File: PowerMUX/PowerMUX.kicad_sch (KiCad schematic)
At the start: 28 parts, among them J1 Conn_01x02_Pin, J2 UJ31-CH-G2-SMT-TR, U1 FT230XS-R, U2 LM2596S-5, U3 TPS2115APW, U4 LM3940IMP-3.3

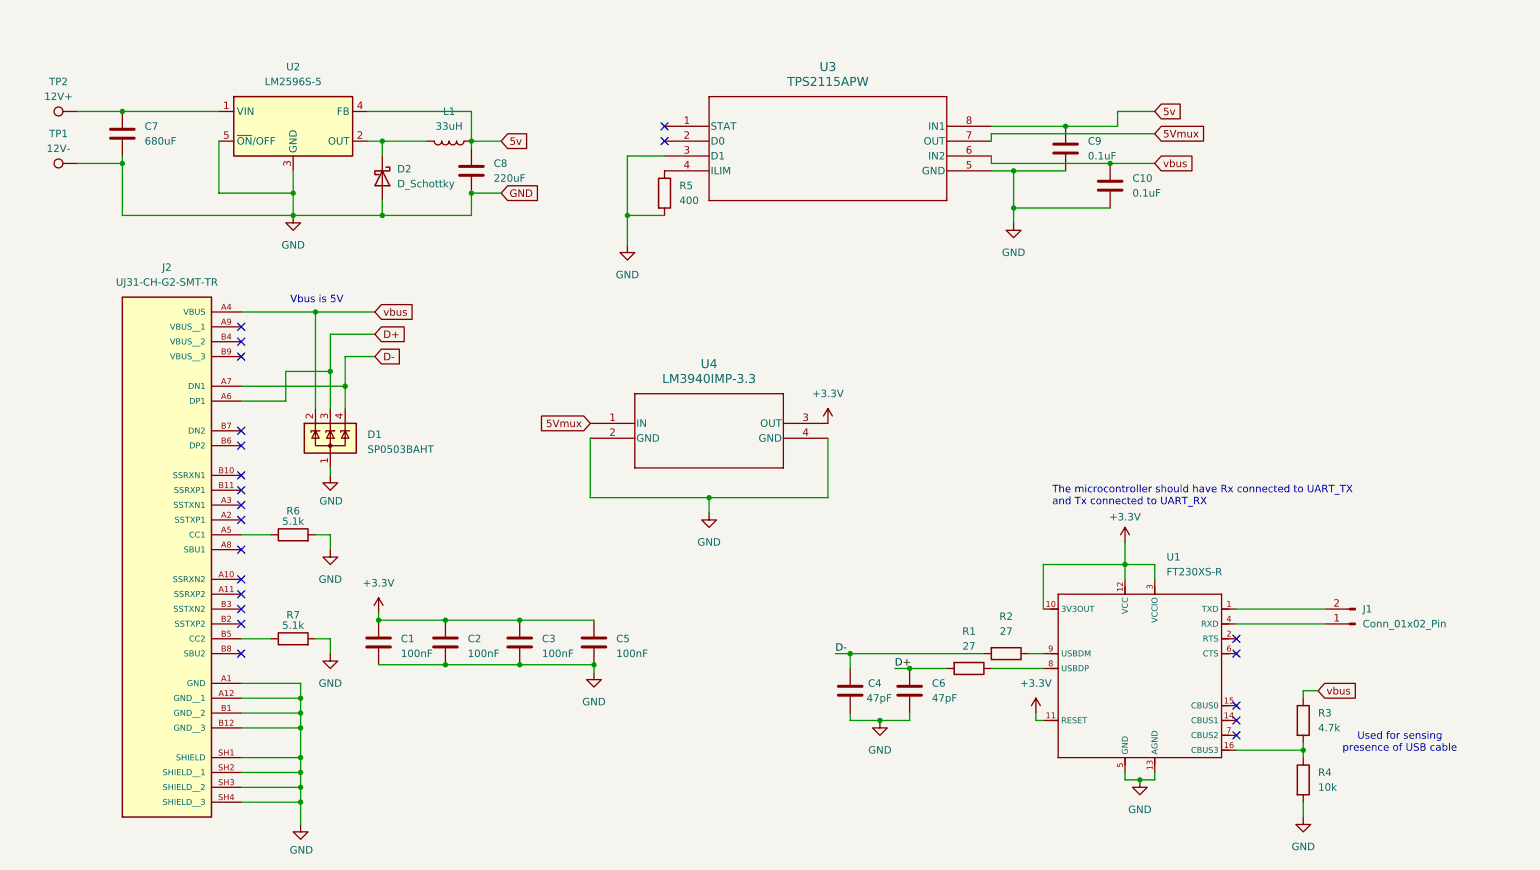
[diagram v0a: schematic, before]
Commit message: changed old THT buck converter to SMD buck converter from LSOM
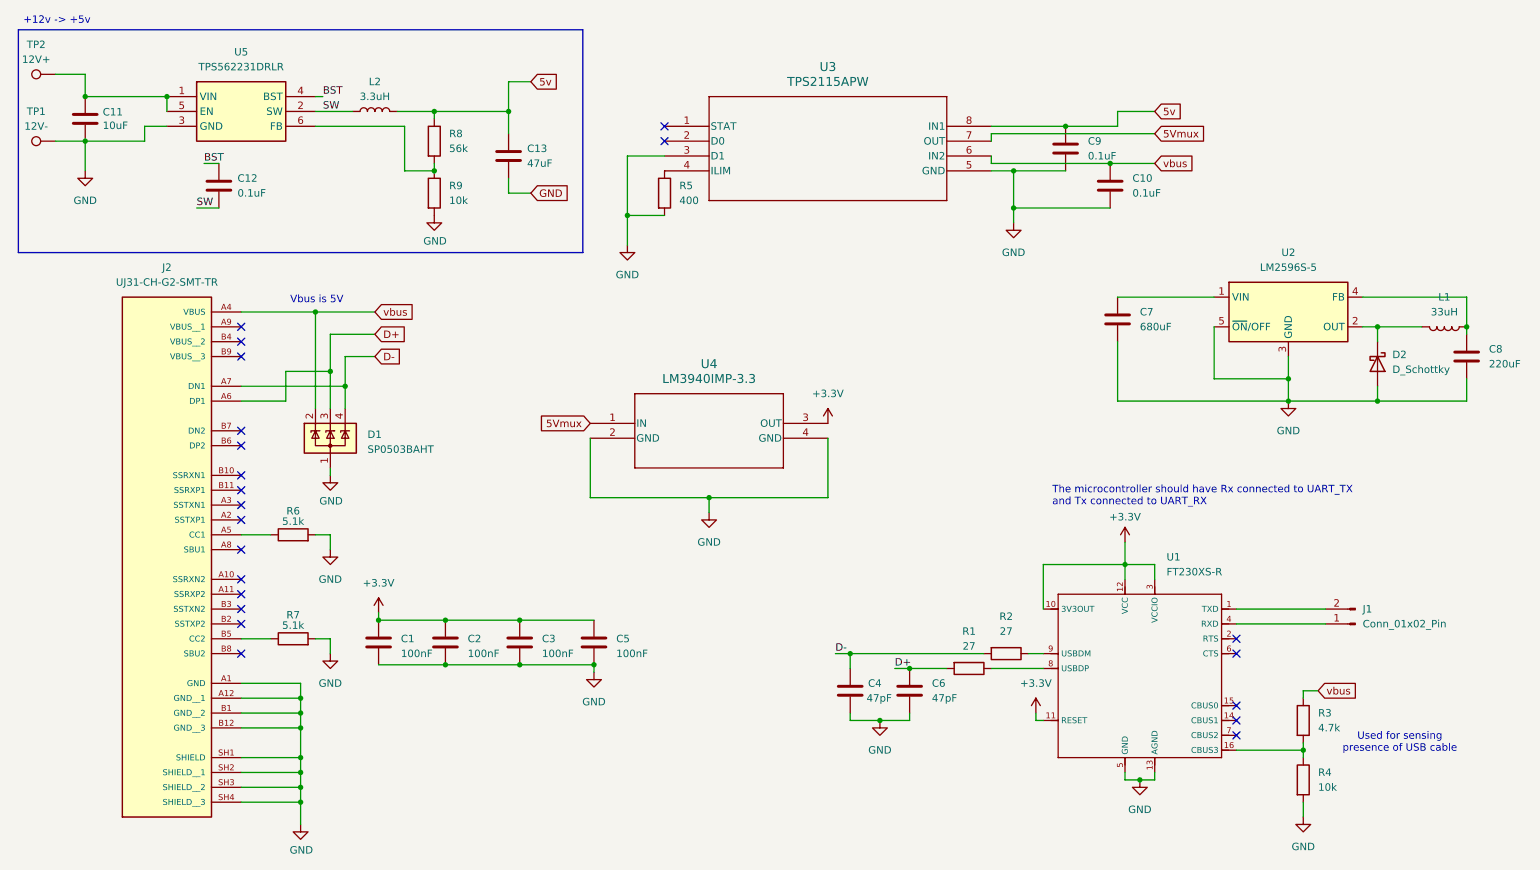
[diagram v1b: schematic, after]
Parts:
- added C11: 10uF, Capacitor_SMD:C_0805_2012Metric, symbol Device:C
- added C12: 0.1uF, Capacitor_SMD:C_0805_2012Metric, symbol Device:C
- added C13: 47uF, Capacitor_SMD:C_0805_2012Metric, symbol Device:C
- added L2: 3.3uH, Inductor_SMD:L_0805_2012Metric_Pad1.15x1.40mm_HandSolder, symbol Device:L
- added R8: 56k, Resistor_SMD:R_0805_2012Metric, symbol Device:R
- added R9: 10k, Resistor_SMD:R_0805_2012Metric, symbol Device:R
- added U5: TPS562231DRLR, Package_TO_SOT_SMD:SOT-563, symbol utsvt-power-regulators:TPS562231DRLR
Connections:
- net 5v: now also C13.1, L2.2, R8.1; no longer C8.1, L1.1, U2.4 (FB)
- net GND: now also C11.2, C13.2, R9.2, U5.3 (GND)
- net at C7.1, U2.1 (VIN): no longer TP2.1
- new net: R8.2, R9.1, U5.6 (FB)
- new net: C11.1, TP2.1, U5.1 (VIN), U5.5 (EN)
- new net: C8.1, L1.1, U2.4 (FB)
- new net BST: C12.1, U5.4 (BST)
- new net SW: C12.2, L2.1, U5.2 (SW)
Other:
- note added: "+12v -> +5v"
- moved on the sheet: C7, C8, D2, L1, TP1, TP2, U2
